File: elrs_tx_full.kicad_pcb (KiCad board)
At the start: 2 copper layers, 31.4 x 66.3 mm, 11 parts, among them J1 LED Chain, J2 DEBUG, J3 RUN, J4 DC_DC, J5 OLED_I2C, U1 E28-2G4M27S-MY, U2 ESP32-WROOM-32-MY

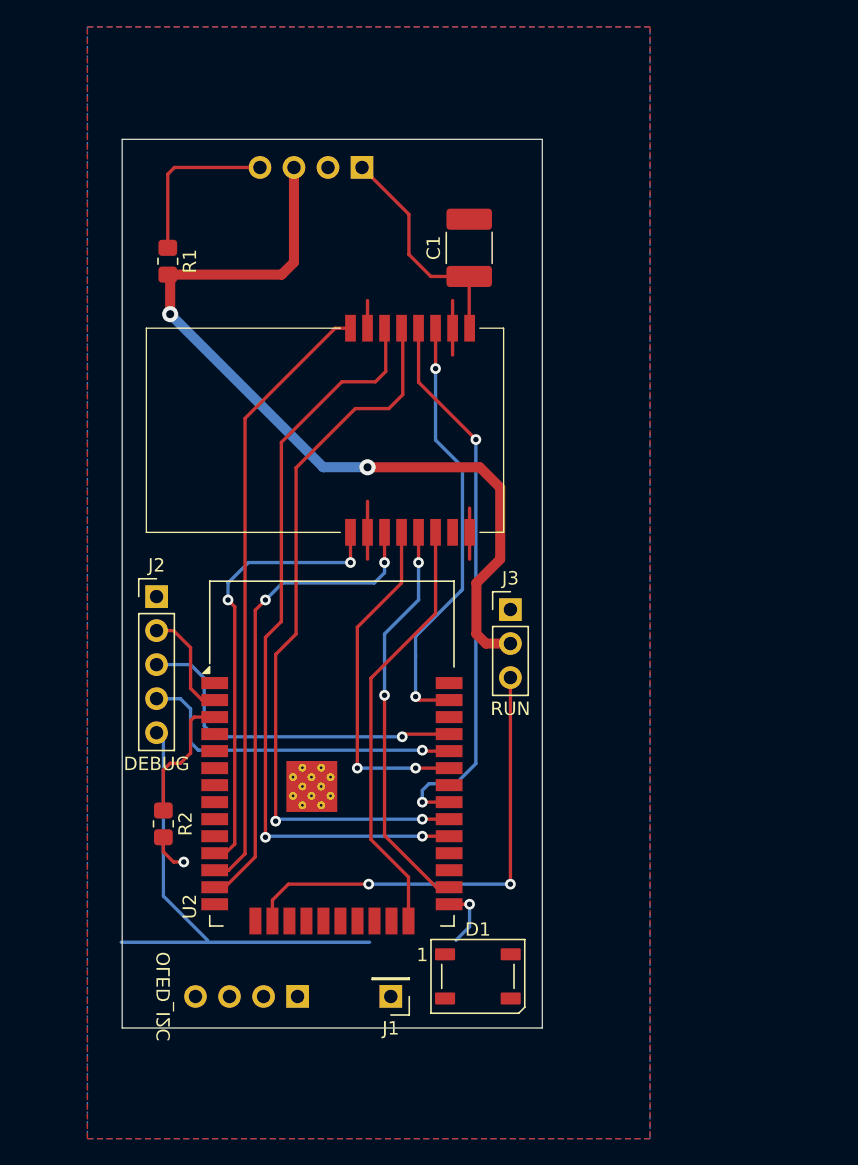
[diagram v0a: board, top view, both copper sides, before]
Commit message: pcb progress
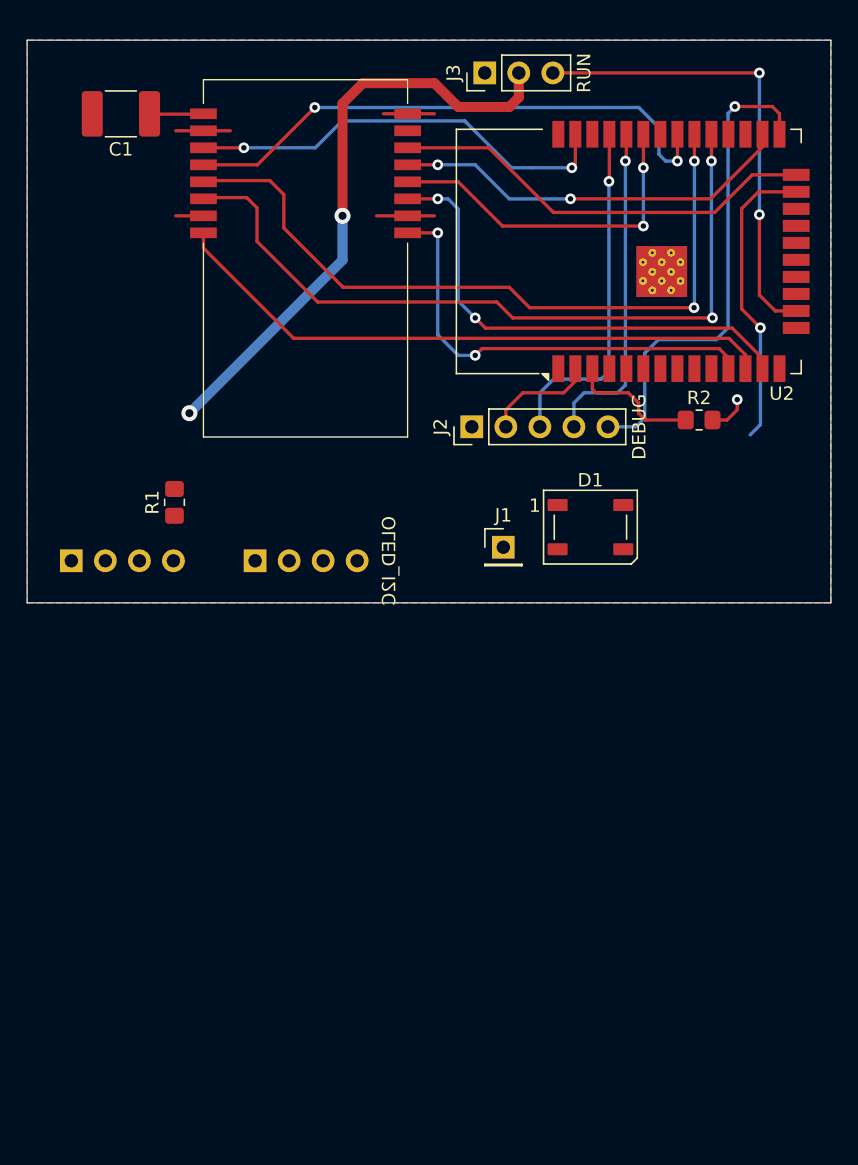
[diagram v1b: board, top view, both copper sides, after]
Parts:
- J4: footprint Connector_PinHeader_2.54mm:PinHeader_1x04_P2.54mm_Vertical -> elrs_tx_full:DC_DC_20x11
- moved R2 50.1 mm to (130.2, 68.4), turned to 0 degrees
- moved U2 47.6 mm to (127.9, 55.8), turned to 90 degrees
- moved J3 40.1 mm to (114.2, 42.4), turned to 90 degrees
- moved J4 36.5 mm to (83.3, 78.9), turned to -90 degrees
- moved D1 34.6 mm to (122.0, 76.3)
- moved J1 34.6 mm to (115.5, 77.8), turned to 0 degrees
- moved J5 32.7 mm to (97.0, 78.9), turned to -90 degrees
- moved C1 27.9 mm to (87.0, 45.5), turned to 180 degrees
- moved J2 26.7 mm to (113.2, 68.9), turned to 90 degrees
- moved R1 18.0 mm to (91.0, 74.5), turned to 90 degrees
- moved U1 13.6 mm to (100.8, 55.7), turned to 180 degrees
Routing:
- net /LED_RGB: track 0.00 -> 22.4 mm, vias 0 -> 1
- net +BATT: track 64.4 -> 44.5 mm
- net +3.3V: track 28.2 -> 15.1 mm
- net Net-(J4-Pin_4): track 12.6 -> 0.00 mm
- net /ESP32_BOOT0: track 40.3 -> 36.7 mm
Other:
- board size 31.4 x 66.3 mm -> 60 x 42 mm

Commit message: pcb progress
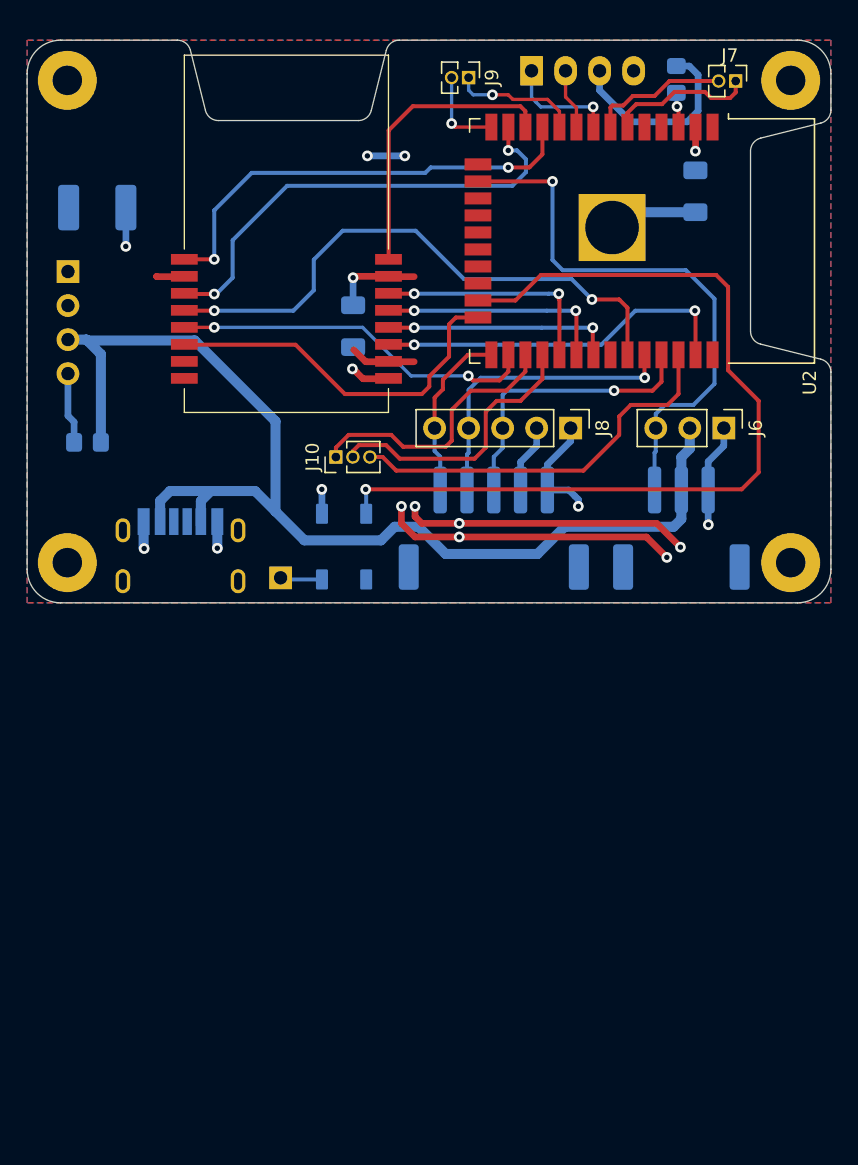
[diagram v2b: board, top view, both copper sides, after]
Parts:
- added C2: 10uF, Capacitor_SMD:C_1206_3216Metric_Pad1.33x1.80mm_HandSolder, B.Cu at (129.9, 51.3)
- added C3: 10uF, Capacitor_SMD:C_1206_3216Metric_Pad1.33x1.80mm_HandSolder, B.Cu at (104.3, 61.3)
- added H1: MountingHole, MountingHole:MountingHole_2.2mm_M2_Pad, F.Cu at (83.0, 43.0)
- added H2: MountingHole, MountingHole:MountingHole_2.2mm_M2_Pad, F.Cu at (83.0, 79.0)
- added H3: MountingHole, MountingHole:MountingHole_2.2mm_M2_Pad, F.Cu at (137.0, 43.0)
- added H4: MountingHole, MountingHole:MountingHole_2.2mm_M2_Pad, F.Cu at (137.0, 79.0)
- added J10: IO3, Connector_PinHeader_1.27mm:PinHeader_1x03_P1.27mm_Vertical, F.Cu at (103.0, 71.1)
- added J6: RUN, Connector_PinHeader_2.54mm:PinHeader_1x03_P2.54mm_Vertical, F.Cu at (132.0, 69.0)
- added J7: IO1, Connector_PinHeader_1.27mm:PinHeader_1x02_P1.27mm_Vertical, F.Cu at (132.9, 43.0)
- added J8: DEBUG, Connector_PinHeader_2.54mm:PinHeader_1x05_P2.54mm_Vertical, F.Cu at (120.6, 69.0)
- added J9: IO2, Connector_PinHeader_1.27mm:PinHeader_1x02_P1.27mm_Vertical, F.Cu at (113.0, 42.8)
- added P1: USB_C_Plug_USB2.0, elrs_tx_full:USB_C_DEALON_009, B.Cu at (91.4, 76.3)
- C1, D1, J1, R1, R2: moved to B.Cu
- J2: footprint Connector_PinHeader_2.54mm:PinHeader_1x05_P2.54mm_Vertical -> Connector_JST:JST_PH_S5B-PH-SM4-TB_1x05-1MP_P2.00mm_Horizontal; moved to B.Cu
- J3: footprint Connector_PinHeader_2.54mm:PinHeader_1x03_P2.54mm_Vertical -> Connector_JST:JST_PH_S3B-PH-SM4-TB_1x03-1MP_P2.00mm_Horizontal; moved to B.Cu
- J5: footprint Connector_PinHeader_2.54mm:PinHeader_1x04_P2.54mm_Vertical -> elrs_tx_full:OLED_27.3x27.8mm_no_holes
- U2: footprint elrs_tx_full:ESP32-WROOM-32D-MY -> elrs_tx_full:ESP32-WROOM-32_zhaw
- moved J5 44.0 mm to (121.5, 42.3), turned to 180 degrees
- moved J3 37.0 mm to (128.8, 76.4), turned to 180 degrees
- moved R2 25.5 mm to (128.5, 42.9), turned to 90 degrees
- moved J4 21.6 mm to (83.0, 57.3), turned to 180 degrees
- moved D1 18.4 mm to (103.7, 77.8), turned to 90 degrees
- moved J1 16.8 mm to (98.9, 80.1), turned to 180 degrees
- moved R1 7.89 mm to (84.5, 70.0), turned to 0 degrees
- moved J2 7.74 mm to (114.8, 76.4), turned to 180 degrees
- moved C1 7.22 mm to (85.2, 52.5), turned to 0 degrees
- moved U2 5.05 mm to (122.9, 55.0), turned to -90 degrees
- moved U1 1.53 mm to (99.4, 55.1), turned to 0 degrees
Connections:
- U2 pad 10: unconnected-(U2-IO25-Pad10) -> /IO25
- U2 pad 14: unconnected-(U2-IO12-Pad14) -> /IO12
- U2 pad 27: unconnected-(U2-IO16-Pad27) -> /IO16
- U2 pad 28: unconnected-(U2-IO17-Pad28) -> /IO17
- U2 pad 36: unconnected-(U2-IO22-Pad36) -> /IO22
- U2 pad 6: unconnected-(U2-IO34-Pad6) -> /IO34
- U2 pad 7: unconnected-(U2-IO35-Pad7) -> /IO35
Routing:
- net +3.3V: track 15.1 -> 68.8 mm, vias 1 -> 8
- net /LED_RGB: track 22.4 -> 66.3 mm
- net +BATT: track 44.5 -> 87.8 mm, vias 2 -> 0
- net /E28_NSS_CTS: track 57.0 -> 17.3 mm
- net /E28_SCK_RTS: track 55.0 -> 17.3 mm
- net GND: track 14.3 -> 47.4 mm, vias 0 -> 9
- net /IO22: track 0.00 -> 29.6 mm
- net /E28_MISO_RX: track 42.0 -> 17.3 mm
- net /E28_RX_EN: track 45.9 -> 21.9 mm
- net /ESP32_BOOT0: track 36.7 -> 13.0 mm, vias 1 -> 0
- net /IO17: track 0.00 -> 21.0 mm
- net /IO16: track 0.00 -> 20.5 mm
- net /E28_BUSY: track 25.8 -> 42.8 mm
- net /IO34: track 0.00 -> 11.0 mm
- net /IO35: track 0.00 -> 10.4 mm
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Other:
- outline, holes or cut-outs redrawn

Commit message: pcb progress
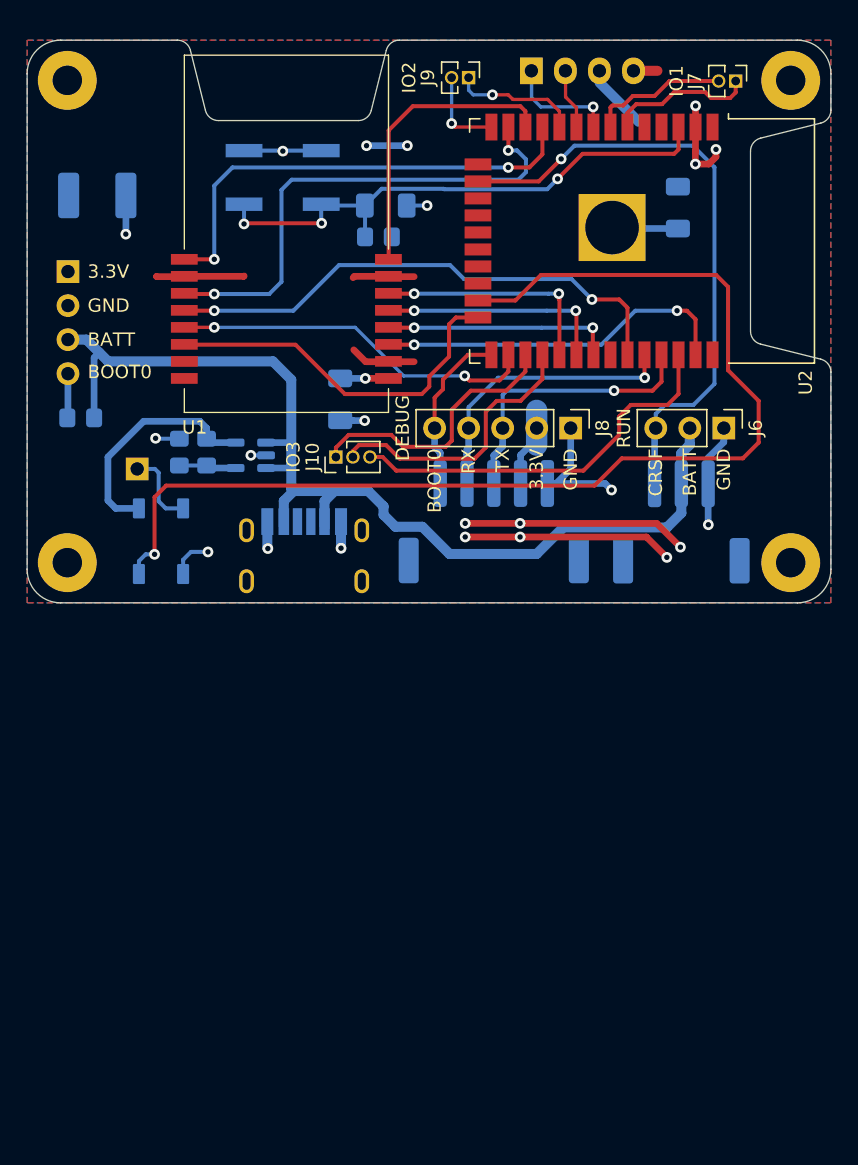
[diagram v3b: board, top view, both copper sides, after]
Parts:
- added C9: 10uF, Capacitor_SMD:C_1206_3216Metric_Pad1.33x1.80mm_HandSolder, B.Cu at (106.8, 52.3)
- added R3: 56k, Resistor_SMD:R_0805_2012Metric_Pad1.20x1.40mm_HandSolder, B.Cu at (93.4, 70.8)
- added R4: 22k, Resistor_SMD:R_0805_2012Metric_Pad1.20x1.40mm_HandSolder, B.Cu at (91.4, 70.8)
- added SW1: RESET, Button_Switch_SMD:SW_SPST_EVQP0, B.Cu at (99.1, 50.2)
- added U3: SPX3819M5-L, Package_TO_SOT_SMD:SOT-23-5, B.Cu at (96.7, 71.0)
- moved R2 25.2 mm to (106.2, 54.7), turned to 0 degrees
- moved D1 13.7 mm to (90.0, 77.4), turned to -90 degrees
- moved J1 13.4 mm to (88.2, 72.0)
- moved P1 9.23 mm to (100.7, 76.3)
- moved C3 5.55 mm to (103.4, 66.8), turned to -90 degrees
- moved R1 1.90 mm to (84.0, 68.2)
- moved C2 1.79 mm to (128.6, 52.5)
- moved C1 0.91 mm to (85.2, 51.6)
- moved J2 0.49 mm to (114.8, 75.9)
- moved J3 0.47 mm to (128.8, 76.0)
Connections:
- net Net-(U2-EN) renamed /EN
- D1 pad 1: +3.3V -> +5V
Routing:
- net /EN: track 2.62 -> 41.2 mm, vias 1 -> 3
- net /LED_RGB: track 66.3 -> 85.8 mm
- net GND: track 47.4 -> 66.4 mm, vias 9 -> 13
- net +5V: track 0.00 -> 17.6 mm
- net +3.3V: track 68.8 -> 55.2 mm, vias 8 -> 10
- net +BATT: track 87.8 -> 80.3 mm
- net /CRSF_RX_TX: track 42.1 -> 46.6 mm
- net Net-(U3-ADJ): track 0.00 -> 4.27 mm
- net /E28_BUSY: track 42.8 -> 39.3 mm
- net /E28_NRESET: track 35.2 -> 37.7 mm
- net Net-(D1-DOUT): track 3.57 -> 5.90 mm
- net Net-(J4-Pin_4): track 5.32 -> 3.32 mm
- net /E28_TX_EN: track 34.2 -> 35.2 mm
- net /ESP32_RX: track 22.8 -> 22.0 mm
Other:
- board text added: "3.3V"
- board text added: "BATT"
- board text added: "BOOT0"
- board text added: "CRSF"
- board text added: "GND"
- board text added: "RX"
- board text added: "SCK"
- board text added: "SDA"
- board text added: "TX"
